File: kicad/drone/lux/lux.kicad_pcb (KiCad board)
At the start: 4 copper layers, 0 parts

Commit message: sept 13
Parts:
- added B1: BL5612, easyeda2kicad:SOP-8_L4.9-W3.9-P1.27-LS6.0-BL, F.Cu at (1151.2, 1044.7)
- added B2: BL5612, easyeda2kicad:SOP-8_L4.9-W3.9-P1.27-LS6.0-BL, F.Cu at (1151.2, 1053.3)
- added B3: BL5612, easyeda2kicad:SOP-8_L4.9-W3.9-P1.27-LS6.0-BL, F.Cu at (1242.5, 1052.8)
- added B4: BL5612, easyeda2kicad:SOP-8_L4.9-W3.9-P1.27-LS6.0-BL, F.Cu at (1242.3, 1043.0)
- added BMP1: BMP180, Connector_Hirose:Hirose_DF13-04P-1.25DSA_1x04_P1.25mm_Vertical, F.Cu at (1169.8, 1040.2)
- added BT1: 600mah, Connector_PinHeader_2.54mm:PinHeader_1x02_P2.54mm_Vertical, F.Cu at (1204.0, 1059.2)
- added C1: 10 uF, Capacitor_SMD:C_0805_2012Metric, F.Cu at (1151.0, 1038.2)
- added C10: 22 uF, Capacitor_SMD:C_1206_3216Metric, F.Cu at (1172.0, 1059.4)
- added C11: 22 uF, Capacitor_SMD:C_1206_3216Metric, F.Cu at (1172.0, 1062.8)
- added C12: 22 uF, Capacitor_SMD:C_1206_3216Metric, F.Cu at (1172.0, 1066.1)
- added C13: 22 uF, Capacitor_SMD:C_1206_3216Metric, F.Cu at (1172.0, 1069.5)
- added C14: 10 uF, Capacitor_SMD:C_0805_2012Metric, F.Cu at (1194.3, 1067.5)
- added C15: 0.1 uF, Capacitor_SMD:C_0402_1005Metric, F.Cu at (1207.8, 1067.5)
- added C16: 0.1 uF, Capacitor_SMD:C_0402_1005Metric, F.Cu at (1179.8, 1040.8)
- added C17: 0.1 uF, Capacitor_SMD:C_0402_1005Metric, F.Cu at (1166.0, 1041.0)
- added C18: 0.1 uF, Capacitor_SMD:C_0402_1005Metric, F.Cu at (1207.8, 1073.5)
- added C19: 10 uF, Capacitor_SMD:C_0805_2012Metric, F.Cu at (1181.0, 1035.8)
- added C2: 10 uF, Capacitor_SMD:C_0805_2012Metric, F.Cu at (1151.0, 1058.2)
- added C20: 22 uF, Capacitor_SMD:C_1206_3216Metric, F.Cu at (1211.8, 1058.5)
- added C21: 22 uF, Capacitor_SMD:C_1206_3216Metric, F.Cu at (1220.0, 1058.5)
- added C22: 22 uF, Capacitor_SMD:C_1206_3216Metric, F.Cu at (1224.0, 1058.5)
- added C23: 22 uF, Capacitor_SMD:C_1206_3216Metric, F.Cu at (1215.8, 1058.5)
- added C3: 10 uF, Capacitor_SMD:C_0805_2012Metric, F.Cu at (1242.5, 1058.0)
- added C4: 10 uF, Capacitor_SMD:C_0805_2012Metric, F.Cu at (1242.5, 1038.0)
- added C5: 22 uF, Capacitor_SMD:C_1206_3216Metric, F.Cu at (1151.0, 1035.2)
- added C6: 22 uF, Capacitor_SMD:C_1206_3216Metric, F.Cu at (1151.0, 1060.8)
- added C7: 22 uF, Capacitor_SMD:C_1206_3216Metric, F.Cu at (1242.5, 1060.8)
- added C8: 22 uF, Capacitor_SMD:C_1206_3216Metric, F.Cu at (1242.5, 1035.5)
- added C9: 22 uF, Capacitor_SMD:C_1206_3216Metric, F.Cu at (1166.3, 1072.8)
- added L1: 1.5 uH, Inductor_SMD:L_Bourns-SRN8040_8x8.15mm, F.Cu at (1232.7, 1048.5)
- added M1: Motor_DC, Connector_JST:JST_PH_B2B-PH-K_1x02_P2.00mm_Vertical, F.Cu at (1159.5, 1036.5)
- added M2: Motor_DC, Connector_JST:JST_PH_B2B-PH-K_1x02_P2.00mm_Vertical, F.Cu at (1160.8, 1058.5)
- added M3: Motor_DC, Connector_JST:JST_PH_B2B-PH-K_1x02_P2.00mm_Vertical, F.Cu at (1230.8, 1057.7)
- added M4: Motor_DC, Connector_JST:JST_PH_B2B-PH-K_1x02_P2.00mm_Vertical, F.Cu at (1230.2, 1037.2)
- added MPU1: MPU6050_BREAKOUT, Connector_Hirose:Hirose_DF13-08P-1.25DSA_1x08_P1.25mm_Vertical, F.Cu at (1175.8, 1040.2)
- added R1: 5.6k, Resistor_SMD:R_0603_1608Metric, F.Cu at (1199.6, 1064.2)
- added R2: 5.6k, Resistor_SMD:R_0603_1608Metric, F.Cu at (1204.4, 1063.2)
- added R3: 560k, Resistor_SMD:R_0603_1608Metric, F.Cu at (1204.4, 1065.7)
- added R4: 100k, Resistor_SMD:R_0603_1608Metric, F.Cu at (1204.4, 1068.2)
- added R5: 10k, Resistor_SMD:R_0603_1608Metric, F.Cu at (1205.8, 1052.6)
- added R6: 10k, Resistor_SMD:R_0603_1608Metric, F.Cu at (1195.9, 1056.0)
- added R7: 10k, Resistor_SMD:R_0603_1608Metric, F.Cu at (1196.8, 1031.0)
- added T1: trace, Capacitor_SMD:C_1206_3216Metric, F.Cu at (1176.8, 1035.5)
- added U1: ESP32-S3-WROOM-1U-N16R8, footprints:ESP32-S3-WROOM-1U_EXP, F.Cu at (1193.1, 1043.9)
- added U2: TPS63020DSJR, footprints:DSJ14_2P85X1P58, F.Cu at (1221.9, 1048.7)
- added USBC1: TYPE-C-31-M-12, easyeda2kicad:USB-C_SMD-TYPE-C-31-M-12_1, F.Cu at (1222.2, 1039.3)
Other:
- board outline added: 100.5 x 28 mm

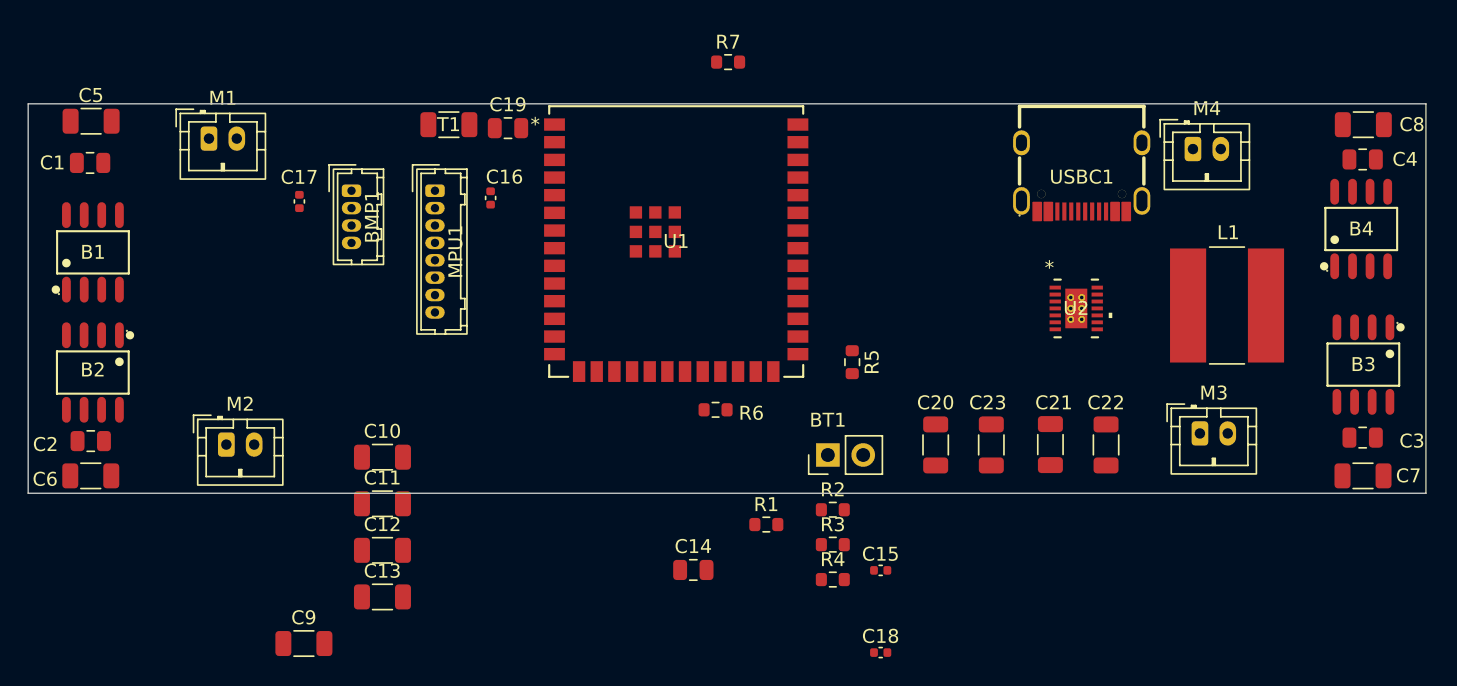
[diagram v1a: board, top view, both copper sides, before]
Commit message: sept 14
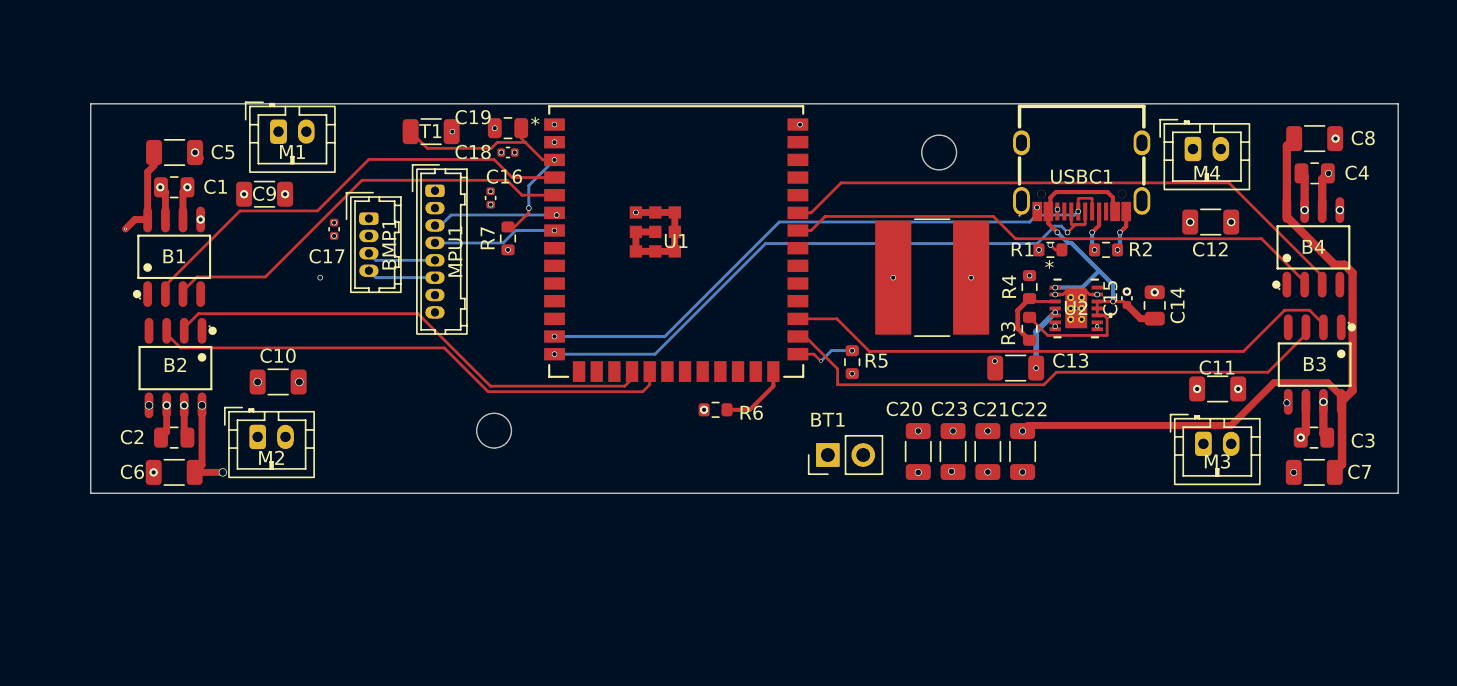
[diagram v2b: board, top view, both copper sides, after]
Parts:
- added H1: MountingHole, MountingHole:MountingHole_2.5mm, F.Cu at (1180.0, 1057.5)
- added H2: MountingHole, MountingHole:MountingHole_2.5mm, F.Cu at (1212.0, 1037.5)
- moved C12 64.1 mm to (1231.5, 1042.5)
- moved C11 60.6 mm to (1232.0, 1054.5)
- moved C13 48.4 mm to (1217.5, 1053.0)
- moved C18 44.8 mm to (1181.0, 1037.5)
- moved C14 38.2 mm to (1227.5, 1048.5), turned to -90 degrees
- moved C9 32.4 mm to (1163.5, 1040.5)
- moved R1 28.4 mm to (1220.0, 1044.5)
- moved R2 27.1 mm to (1224.0, 1044.5), turned to 180 degrees
- moved C15 26.4 mm to (1225.5, 1048.0), turned to 90 degrees
- moved R4 25.3 mm to (1218.5, 1047.2), turned to 90 degrees
- moved L1 21.3 mm to (1211.5, 1046.5)
- moved R3 21.0 mm to (1218.5, 1050.2), turned to 90 degrees
- moved R7 20.3 mm to (1181.0, 1043.7), turned to 90 degrees
- moved C10 9.24 mm to (1164.5, 1054.0)
- moved C5 6.41 mm to (1157.0, 1037.5)
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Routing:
- net +5VA: track 0.00 -> 148.9 mm, vias 0 -> 7
- net +3.3V: track 0.00 -> 96.0 mm, vias 0 -> 12
- net /D+: track 0.00 -> 45.2 mm, vias 0 -> 2
- net /D-: track 0.00 -> 44.2 mm, vias 0 -> 2
- net /IO42: track 0.00 -> 42.0 mm
- net /IO36: track 0.00 -> 40.6 mm
- net /IO35: track 0.00 -> 40.6 mm
- net /IO41: track 0.00 -> 39.0 mm
- net /IO11: track 0.00 -> 37.8 mm
- net /IO10: track 0.00 -> 35.7 mm
- net +5V: track 0.00 -> 32.9 mm, vias 0 -> 3
- net /IO4: track 0.00 -> 32.9 mm
- net /IO5: track 0.00 -> 30.7 mm
- net GND: track 0.00 -> 26.6 mm, vias 0 -> 29
- net /M2B: track 0.00 -> 19.9 mm, vias 0 -> 2
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- added copper zone on In2.Cu, net GND
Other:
- board size 100.5 x 28 mm -> 94 x 28 mm
